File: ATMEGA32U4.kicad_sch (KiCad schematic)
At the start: 4 parts, among them U2 ATMEGA32U4-AU, U3 MIC5219-3_3YM5-TR

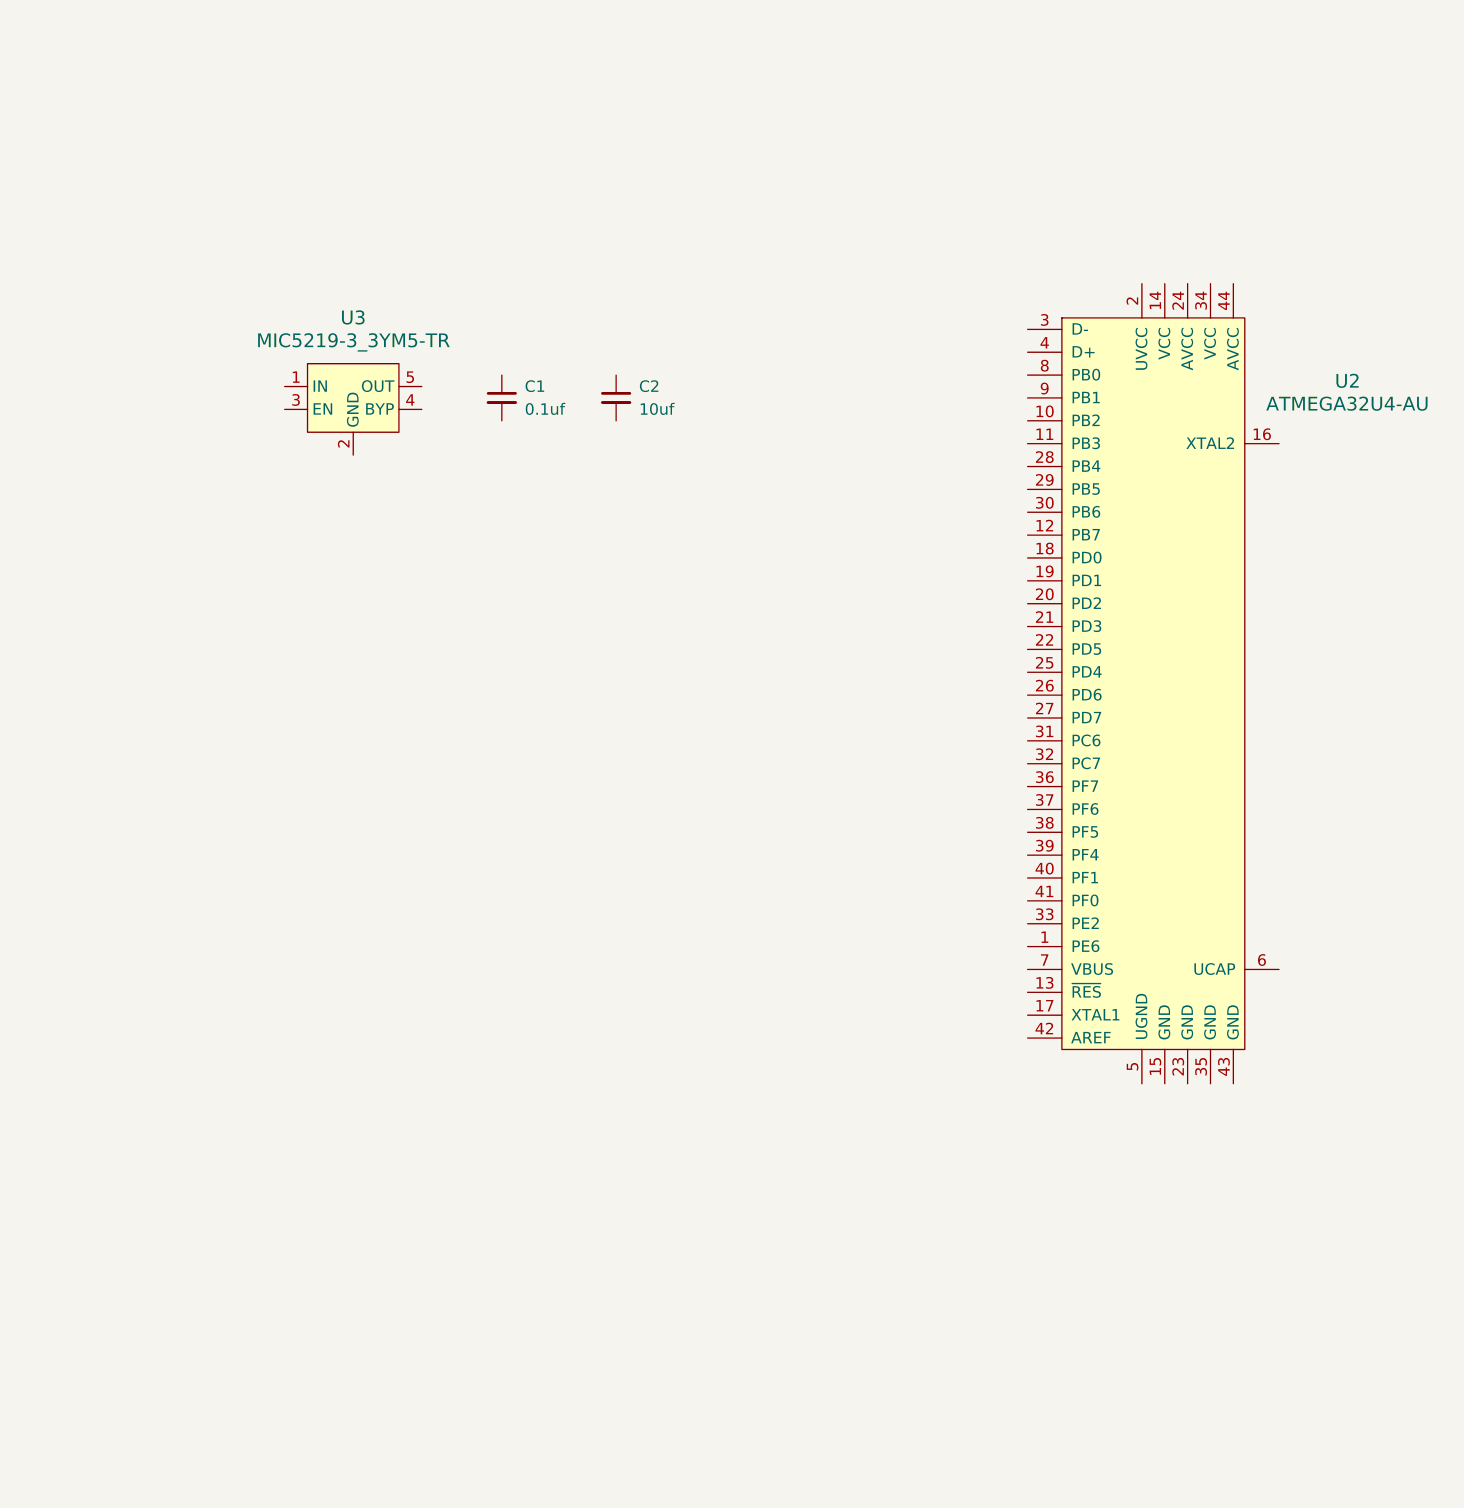
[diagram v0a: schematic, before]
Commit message: improvements
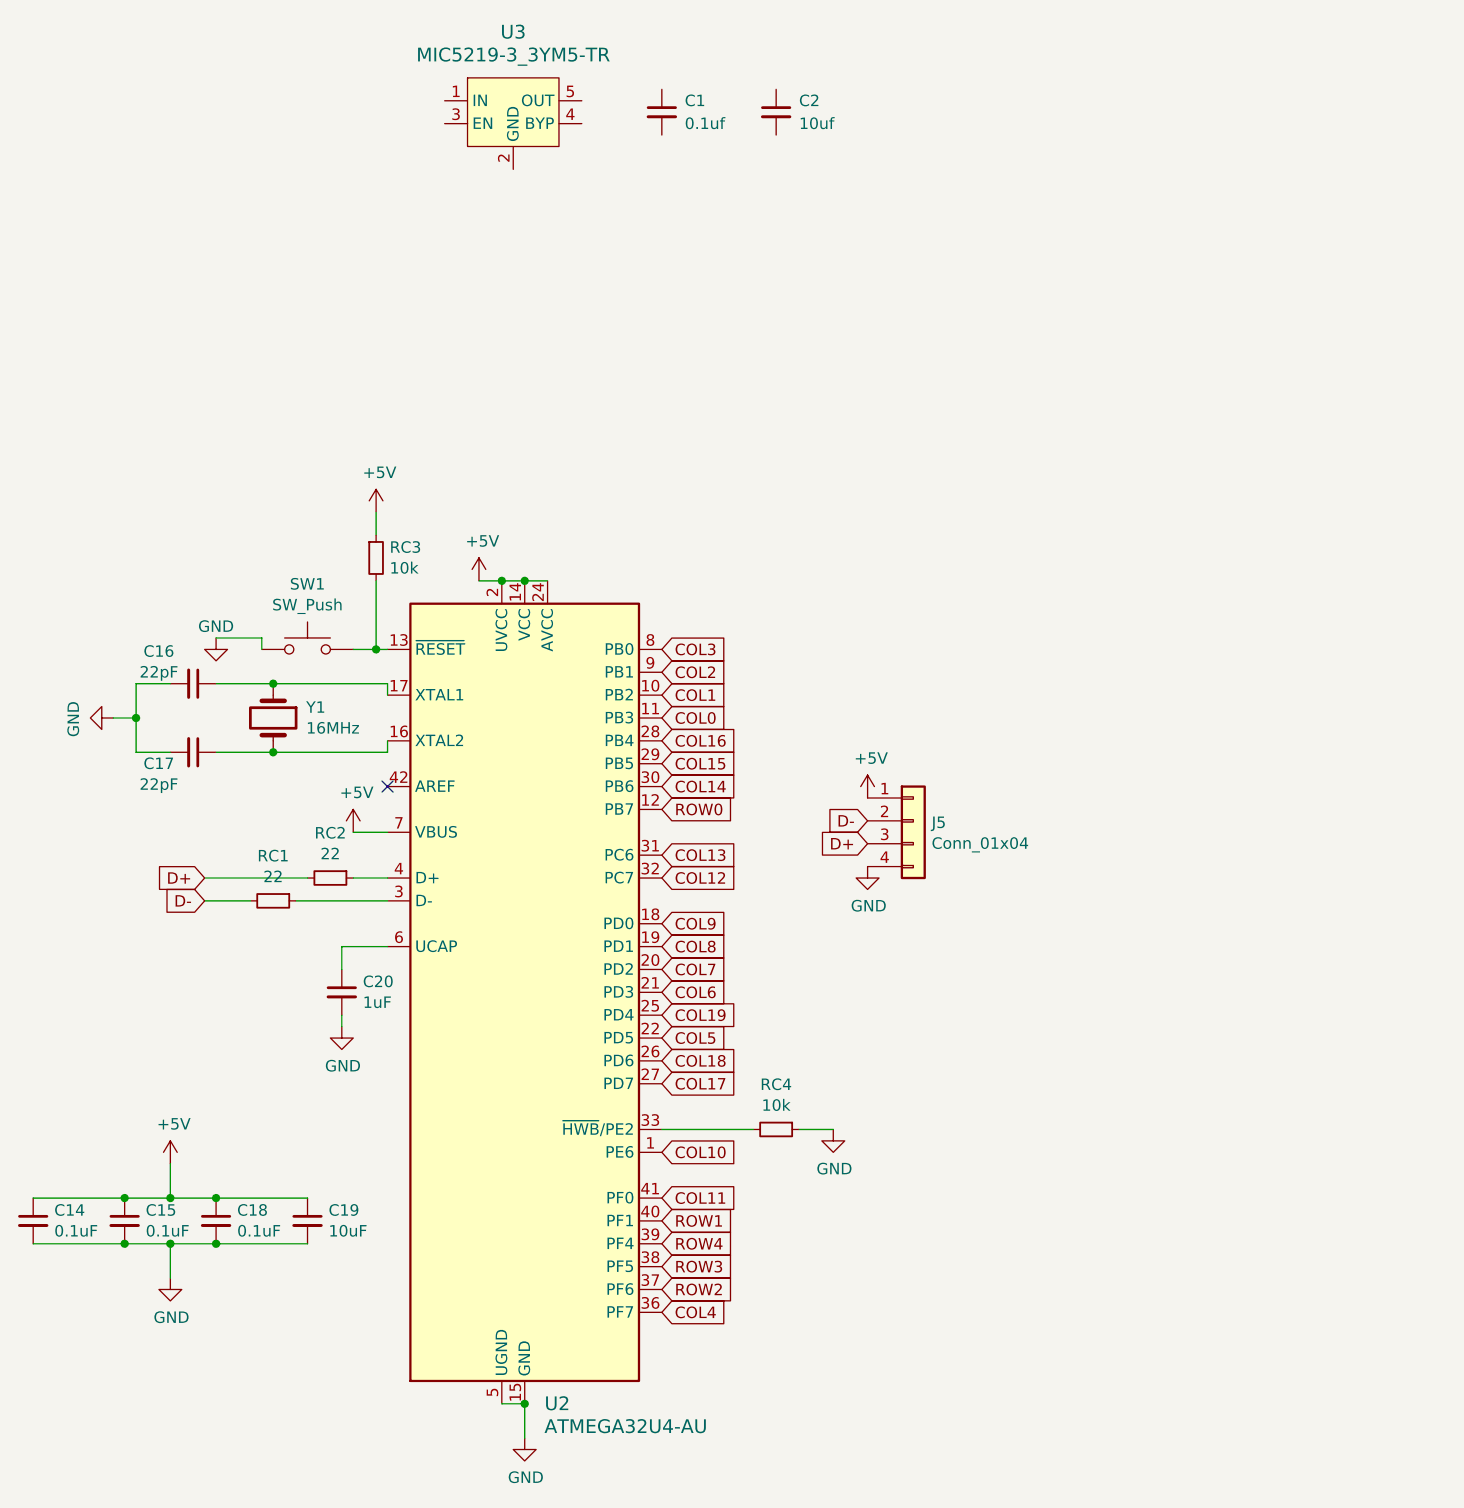
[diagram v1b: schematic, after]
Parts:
- added C14, C15, C18: 0.1uF, Capacitor_SMD:C_0805_2012Metric, symbol Device:C_Small
- added C16, C17: 22pF, Capacitor_SMD:C_0805_2012Metric, symbol Device:C_Small
- added C19: 10uF, Capacitor_SMD:C_0805_2012Metric, symbol Device:C_Small
- added C20: 1uF, Capacitor_SMD:C_0805_2012Metric, symbol Device:C_Small
- added J5: Conn_01x04, random-keyboard-parts:JST-SR-4, symbol Connector_Generic:Conn_01x04
- added RC1, RC2: 22, Resistor_SMD:R_0805_2012Metric, symbol Device:R_Small
- added RC3, RC4: 10k, Resistor_SMD:R_0805_2012Metric, symbol Device:R_Small
- added SW1: SW_Push, Button_Switch_SMD:SW_SPST_PTS645, symbol Switch:SW_Push
- added Y1: 16MHz, Crystal:Crystal_SMD_HC49-SD, symbol Device:Crystal
- U2: footprint digikey-footprints:TQFP-44_10x10mm -> Package_DFN_QFN:QFN-44-1EP_7x7mm_P0.5mm_EP5.2x5.2mm; symbol dk_Embedded-Microcontrollers:ATMEGA32U4-AU -> MCU_Microchip_ATmega:ATmega32U4-M
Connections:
- net COL10: now reaches U2.1 (PE6)
- net COL1: now reaches U2.10 (PB2)
- net COL0: now reaches U2.11 (PB3)
- net ROW0: now reaches U2.12 (PB7)
- net at U2.13 (~{RESET}): now also RC3.2, SW1.2
- net +5V: now reaches U2.14 (VCC)
- net +5V: now also U2.2 (UVCC), U2.24 (AVCC), U2.34 (VCC), U2.44 (AVCC), U2.7 (VBUS), C14.1, C15.1, C18.1, C19.1, J5.1 (Pin_1), RC3.1
- net GND: now reaches U2.15 (GND)
- net GND: now also U2.23 (GND), U2.35 (GND), U2.43 (GND), U2.45 (GND), U2.5 (UGND), C14.2, C15.2, C16.2, C17.2, C18.2, C19.2, C20.2, J5.4 (Pin_4), RC4.1, SW1.1
- net at U2.16 (XTAL2): now also C17.1, Y1.2
- net at U2.17 (XTAL1): now also C16.1, Y1.1
- net COL9: now reaches U2.18 (PD0)
- net COL8: now reaches U2.19 (PD1)
- net COL7: now reaches U2.20 (PD2)
- net COL6: now reaches U2.21 (PD3)
- net COL5: now reaches U2.22 (PD5)
- net COL19: now reaches U2.25 (PD4)
- net COL18: now reaches U2.26 (PD6)
- net COL17: now reaches U2.27 (PD7)
- net COL16: now reaches U2.28 (PB4)
- net COL15: now reaches U2.29 (PB5)
- net at U2.3 (D-): now also RC1.1
- net COL14: now reaches U2.30 (PB6)
- net COL13: now reaches U2.31 (PC6)
- net COL12: now reaches U2.32 (PC7)
- net at U2.33 (~{HWB}/PE2): now also RC4.2
- net COL4: now reaches U2.36 (PF7)
- net ROW2: now reaches U2.37 (PF6)
- net ROW3: now reaches U2.38 (PF5)
- net ROW4: now reaches U2.39 (PF4)
- net at U2.4 (D+): now also RC2.1
- net ROW1: now reaches U2.40 (PF1)
- net COL11: now reaches U2.41 (PF0)
- net at U2.6 (UCAP): now also C20.1
- net COL3: now reaches U2.8 (PB0)
- net COL2: now reaches U2.9 (PB1)
- new net D+: J5.3 (Pin_3), RC2.2
- new net D-: J5.2 (Pin_2), RC1.2
- no-connect marks 0 -> 1
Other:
- moved on the sheet: C1, C2, U3
